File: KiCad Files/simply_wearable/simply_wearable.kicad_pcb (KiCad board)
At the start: 2 copper layers, 30 x 52 mm, 13 parts, among them J1 Conn_01x02_Socket, J3 Conn_01x07_Socket, J4 Conn_01x05_Socket, SW1 SW_Push, SW2 SW_Push, U1 nice_nano, U2 ER_OLEDM0.91_1x-I2C

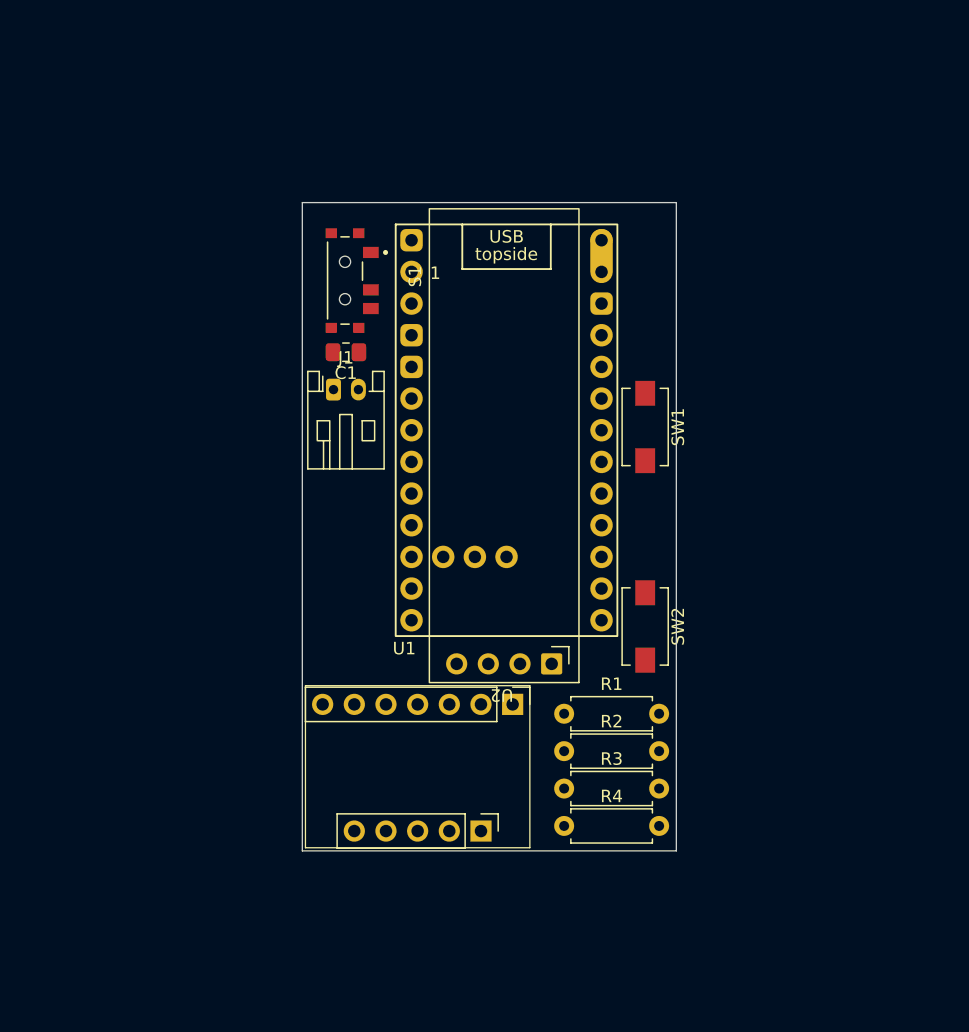
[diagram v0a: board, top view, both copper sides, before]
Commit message: PCB Completed and Production Files Added
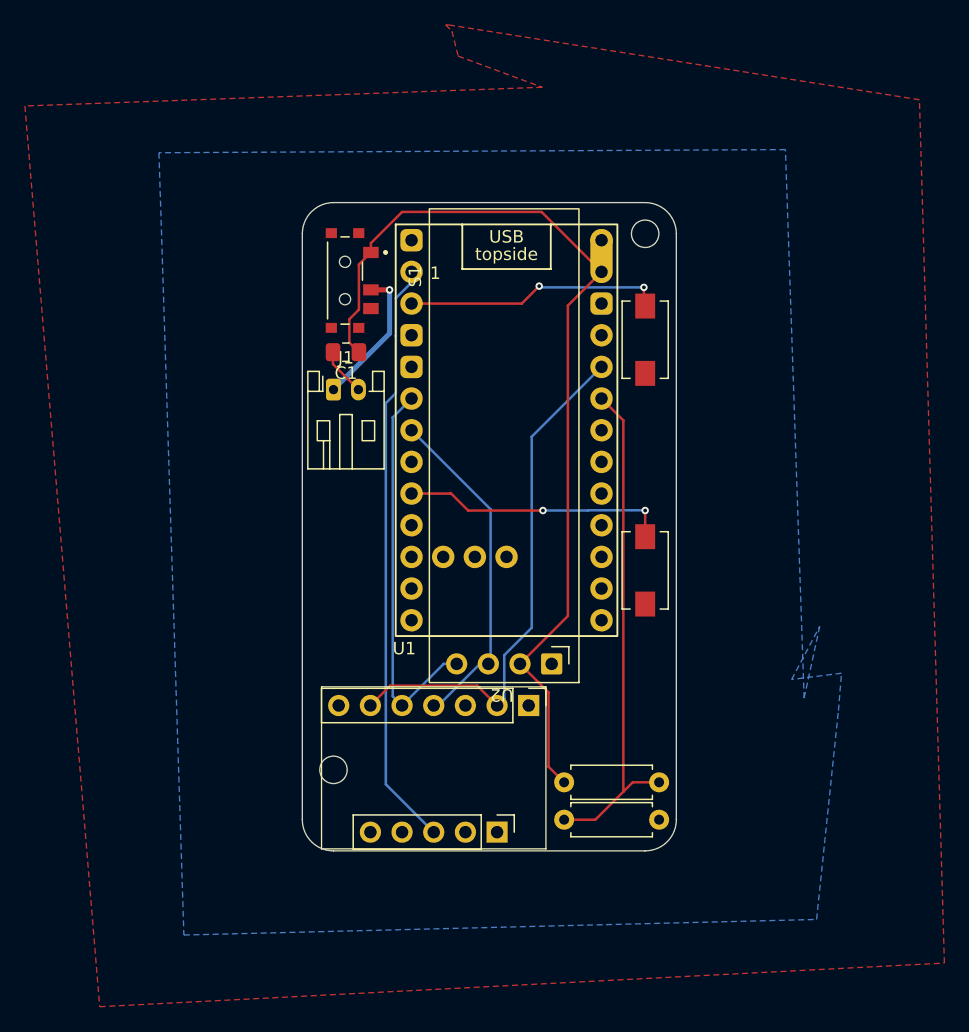
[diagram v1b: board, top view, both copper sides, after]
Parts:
- removed R1: 220, Resistor_THT:R_Axial_DIN0207_L6.3mm_D2.5mm_P7.62mm_Horizontal
- removed R2: 10K, Resistor_THT:R_Axial_DIN0207_L6.3mm_D2.5mm_P7.62mm_Horizontal
- added REF**: MountingHole_2.2mm_M2, MountingHole:MountingHole_2.2mm_M2, F.Cu at (87.5, 76.5)
- added REF**: MountingHole_2.2mm_M2, MountingHole:MountingHole_2.2mm_M2, F.Cu at (112.5, 33.5)
- moved SW1 7.00 mm to (112.5, 42.0)
- moved SW2 4.50 mm to (112.5, 60.5)
- moved J4 1.29 mm to (100.6, 81.5)
- moved J3 1.29 mm to (103.2, 71.3)
- moved R3 0.50 mm to (106.0, 77.5)
- moved R4 0.50 mm to (106.0, 80.5)
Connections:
- U1 pad 29: unconnected-(U1-BAT+-Pad29) -> /VCC
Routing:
- net /VCC: track 0.00 -> 76.4 mm
- net /INT1: track 0.00 -> 47.4 mm
- net /3v3: track 0.00 -> 42.1 mm
- net Net-(U1-P0.31-LF): track 0.00 -> 41.1 mm
- net /SDA: track 0.00 -> 31.3 mm
- net /SCL: track 0.00 -> 27.2 mm
- net /Secondary: track 0.00 -> 21.5 mm, vias 0 -> 2
- net /Primary: track 0.00 -> 20.8 mm, vias 0 -> 2
- net /BAT+: track 0.00 -> 11.4 mm, vias 0 -> 1
- net /GND: track 0.00 -> 3.84 mm
- added copper zone on B.Cu, net /GND
- added copper zone on F.Cu, net /GND
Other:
- outline, holes or cut-outs redrawn
- board text added: ":P"
- board text added: "Aahan Poddar"
- board text added: "Made on Earth by Humans."
- board text added: "simply_wearable"
- board text added: "v1"
